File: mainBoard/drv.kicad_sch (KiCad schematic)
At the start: 6 parts, among them J4 Conn_01x01, J5 Conn_01x01, U3 DRV8251ADDAR

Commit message: Pouzdra
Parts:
- J4, J5: footprint (none) -> Connector_Pin:Pin_D1.0mm_L10.0mm
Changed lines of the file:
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@@
       (effects (font (size 1.27 1.27)) (justify left))
     )
-    (property "Footprint" "" (at 179.07 78.74 0)
+    (property "Footprint" "Connector_Pin:Pin_D1.0mm_L10.0mm" (at 179.07 78.74 0)
       (effects (font (size 1.27 1.27)) hide)
     )
@@
       (effects (font (size 1.27 1.27)) (justify left))
     )
-    (property "Footprint" "" (at 179.07 83.82 0)
+    (property "Footprint" "Connector_Pin:Pin_D1.0mm_L10.0mm" (at 179.07 83.82 0)
       (effects (font (size 1.27 1.27)) hide)
     )

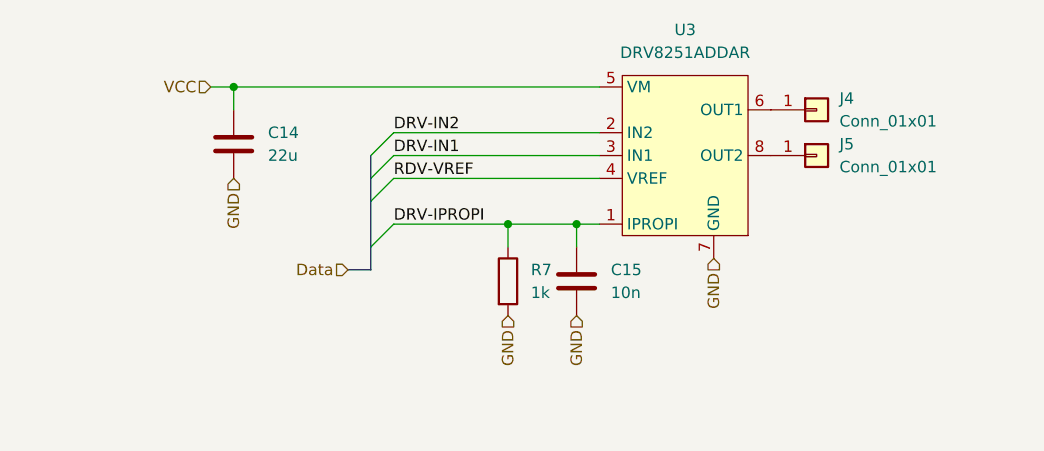
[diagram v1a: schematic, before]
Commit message: test-pointy a zdvojení konektorů
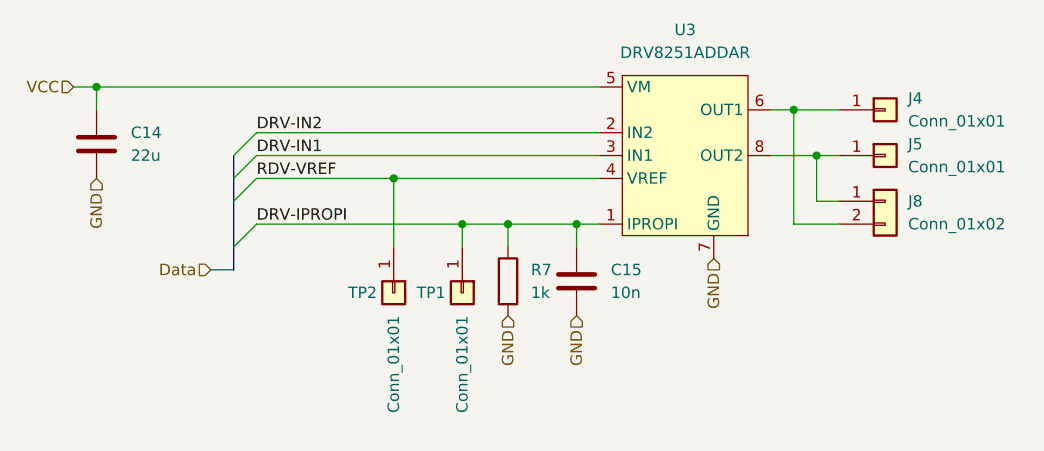
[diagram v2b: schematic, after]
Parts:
- added J8: Conn_01x02, Connector_Phoenix_MC:PhoenixContact_MCV_1,5_2-G-3.81_1x02_P3.81mm_Vertical, symbol Connector_Generic:Conn_01x02
- added TP1, TP2: Conn_01x01, Connector_Pin:Pin_D0.7mm_L6.5mm_W1.8mm_FlatFork, symbol Connector_Generic:Conn_01x01
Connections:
- net DRV-IPROPI: now also TP1.1 (Pin_1)
- net RDV-VREF: now also TP2.1 (Pin_1)
- net at J4.1 (Pin_1), U3.6 (OUT1): now also J8.2 (Pin_2)
- net at J5.1 (Pin_1), U3.8 (OUT2): now also J8.1 (Pin_1)
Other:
- moved on the sheet: C14, J4, J5
